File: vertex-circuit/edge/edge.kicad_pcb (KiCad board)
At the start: 2 copper layers, 60.6 x 52.5 mm, 4 parts

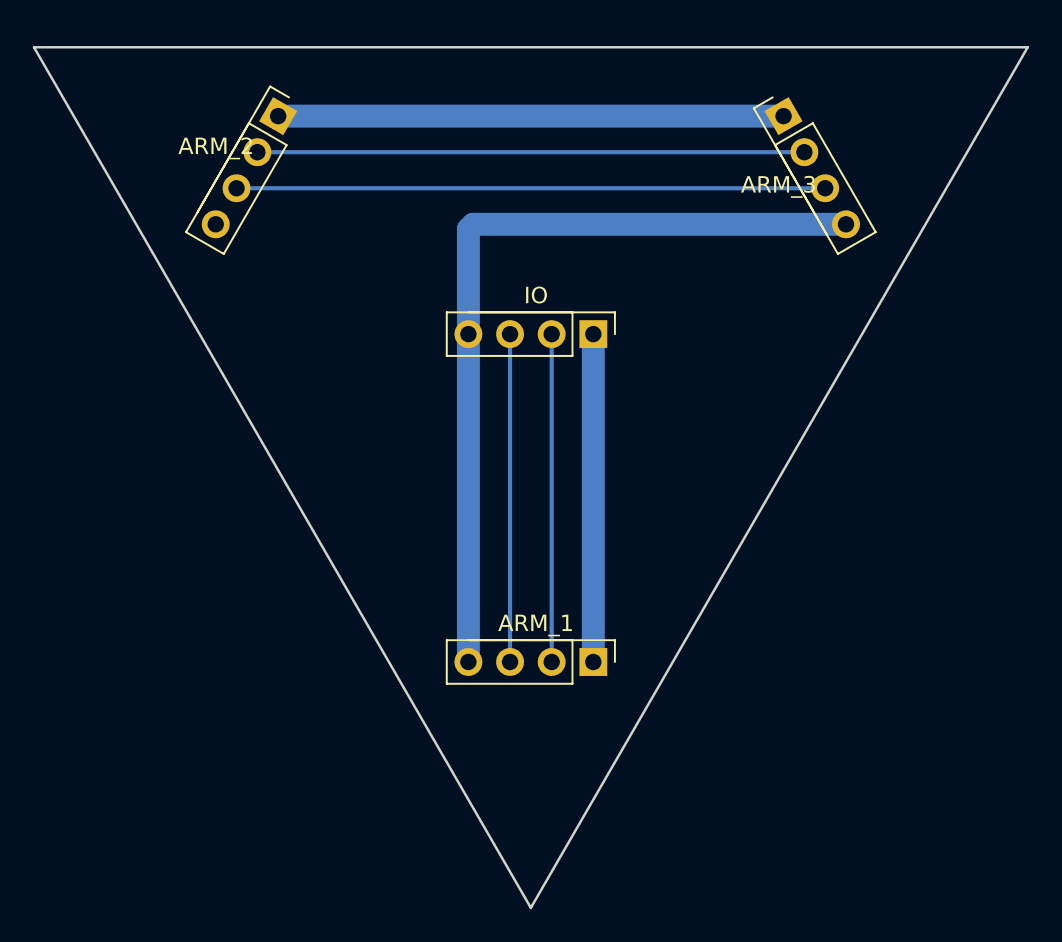
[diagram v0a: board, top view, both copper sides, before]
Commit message: checkpoint
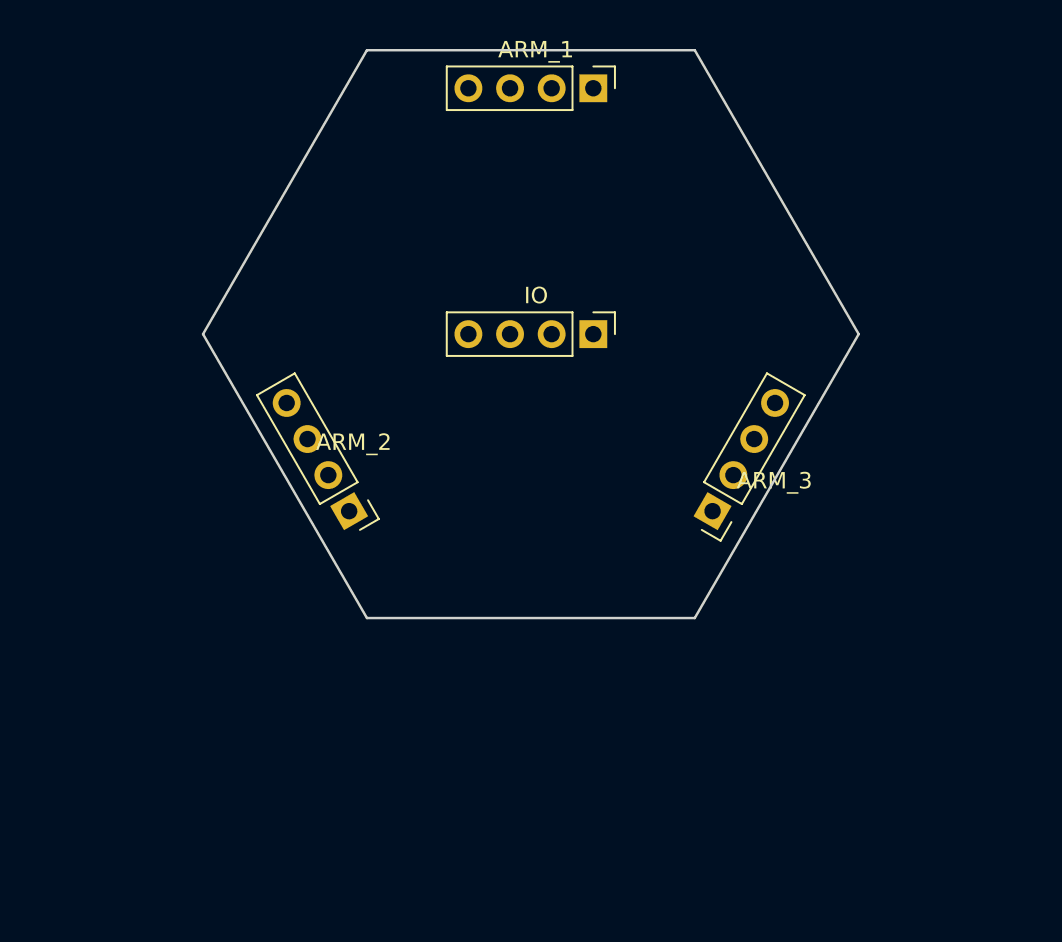
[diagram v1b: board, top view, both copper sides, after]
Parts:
- removed the IO at (150.0, 100.0)
- added IO: H4-2.54mm, H4-2.54mm, F.Cu at (150.0, 100.0)
- ARM_1, ARM_2, ARM_3: footprint PinHeader_1x04_P2.54mm_Vertical_Centered -> H4-2.54mm
- moved ARM_1 35.0 mm to (150.0, 85.0)
- moved ARM_3 18.0 mm to (163.0, 107.5), turned to 150 degrees
- moved ARM_2 18.0 mm to (137.0, 107.5), turned to 210 degrees
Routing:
- net GND: track 50.8 -> 0.00 mm
- net +5V: track 49.6 -> 0.00 mm
- net ARM_2_CLOCK_TO_ARM_3_CLOCK: track 35.9 -> 0.00 mm
- net ARM_2_DATA_TO_ARM_3_DATA: track 33.4 -> 0.00 mm
- net IO_DATA_TO_ARM_1_DATA: track 20.0 -> 0.00 mm
- net IO_CLOCK_TO_ARM_1_CLOCK: track 20.0 -> 0.00 mm
- added copper zone on F.Cu, net GND
- removed copper zone on B.Cu, net GND
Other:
- board size 60.6 x 52.5 mm -> 40 x 34.6 mm
- net class Power: clearance 0.254 -> 0.5; trace_width 1.4 -> 1.7; via_dia 1.4 -> 1.7; via_drill 0.635 -> 0.8
